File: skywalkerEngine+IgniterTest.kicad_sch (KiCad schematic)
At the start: 48 parts

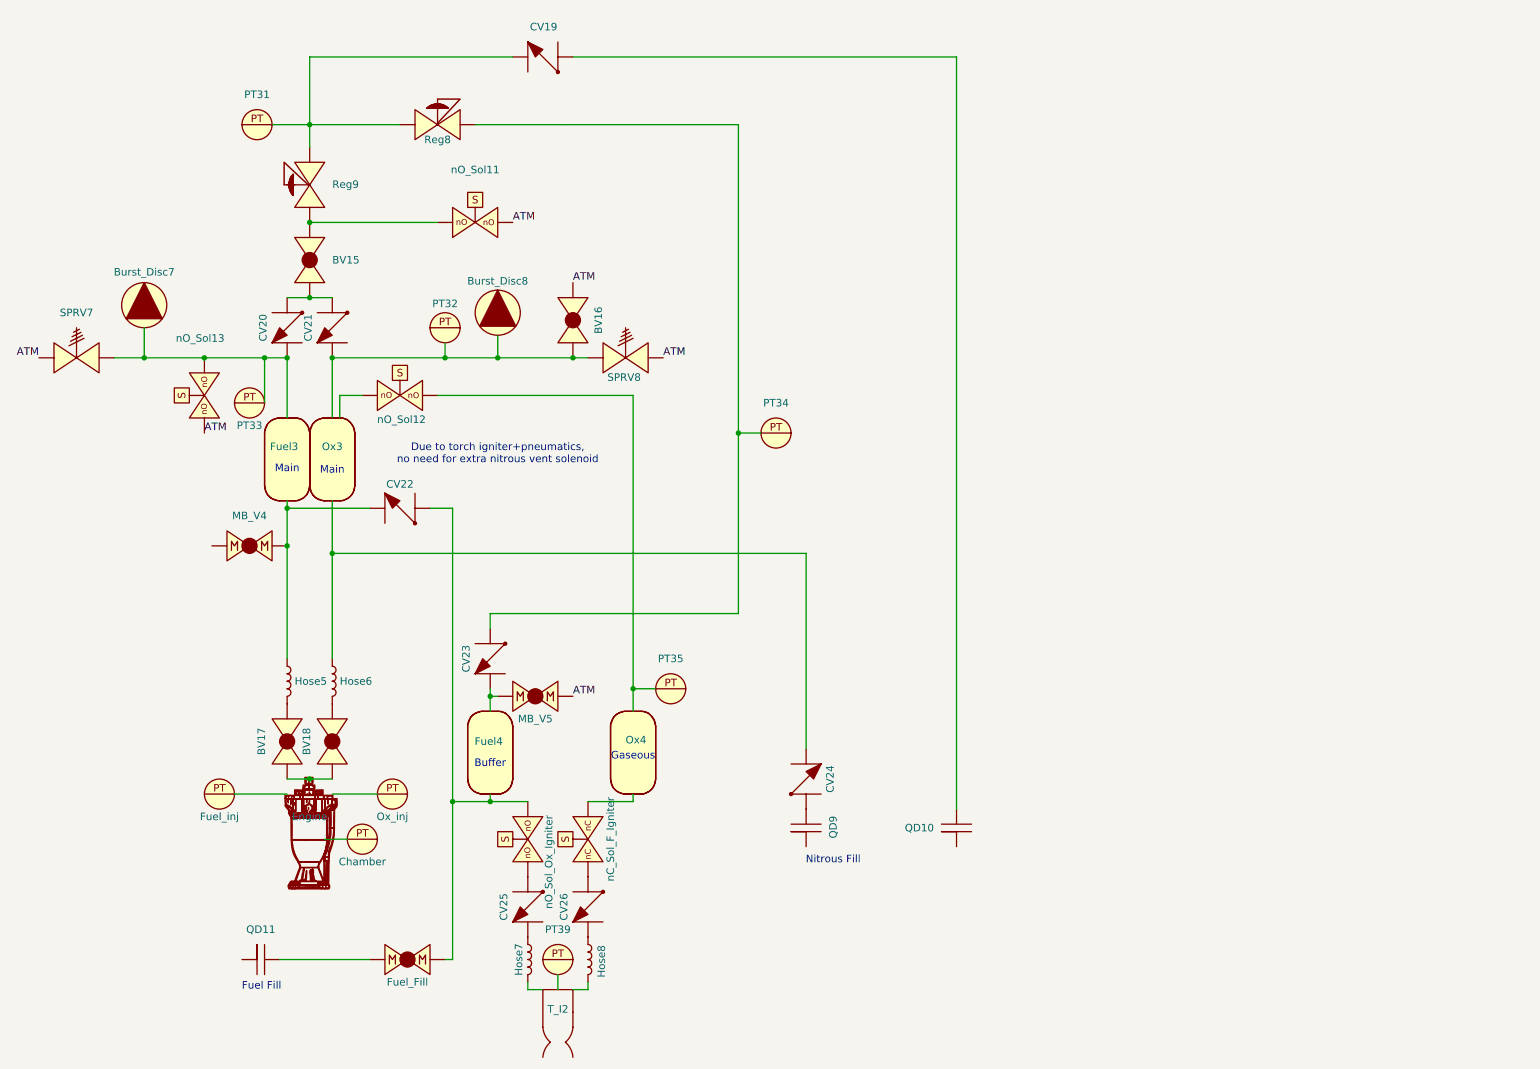
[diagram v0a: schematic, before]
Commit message: overwrite
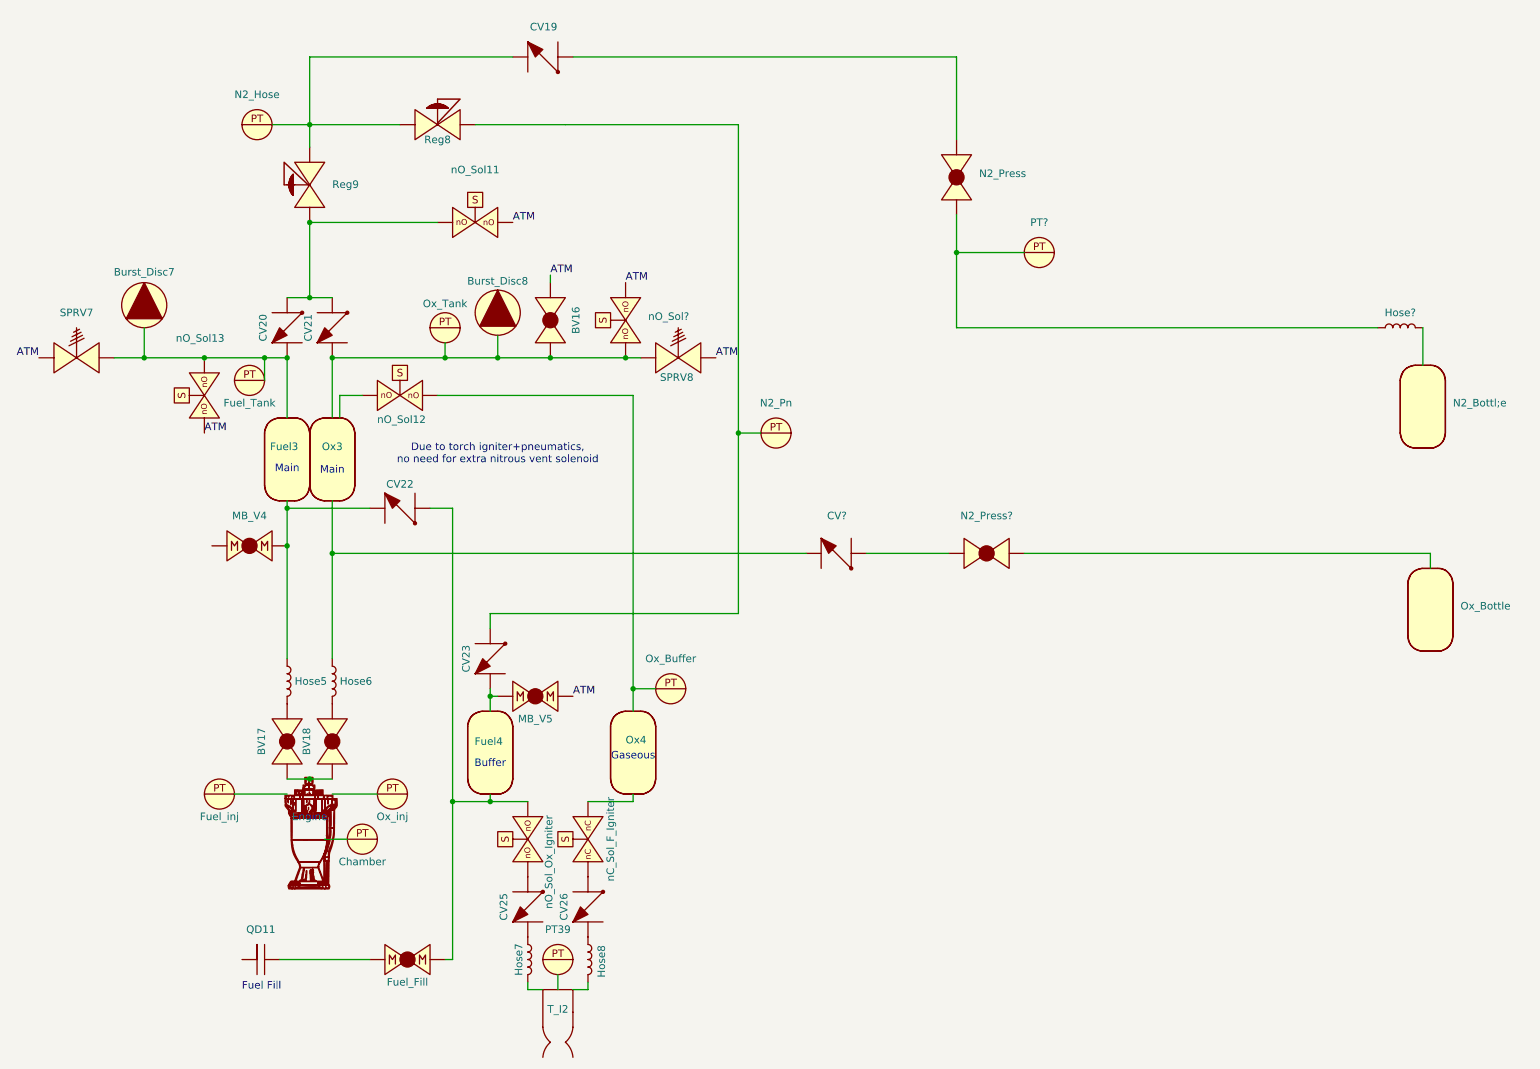
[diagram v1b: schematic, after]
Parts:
- removed BV15: ~, symbol PID_symbols:Ball_Valve
- removed CV24: ~, symbol PID_symbols:Check_Valve
- removed QD10, QD9: ~, symbol PID_symbols:Quick_Disconnect
- added CV?: ~, symbol PID_symbols:Check_Valve
- added Hose?: ~, symbol Device:Hose
- added N2_Bottl;e, Ox_Bottle: ~, symbol PID_symbols:Tank
- added N2_Press, N2_Press?: ~, symbol PID_symbols:Ball_Valve
- added PT?: ~, symbol PID_symbols:Pressure_Transducer
- added nO_Sol?: ~, symbol PID_symbols:Normally Open Solenoid
- renumbered PT33 to Fuel_Tank, PT31 to N2_Hose, PT34 to N2_Pn, PT35 to Ox_Buffer, PT32 to Ox_Tank
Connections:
- net ATM: now also nO_Sol?.
- net at Fuel_inj.: now also Engine.
- net at Engine.: now also Ox_inj.; no longer Fuel_inj.
- net at CV25.: now also Hose7.1; no longer nO_Sol_Ox_Igniter.
- net at CV20., CV21.: now also Reg9., nO_Sol11.
- net at MB_V4.: now also CV22., Fuel3., Hose5.1
- net at Reg9.: now also CV19., N2_Hose., Reg8.; no longer nO_Sol11.
- net at Hose6.1, Ox3.: now also CV?.
- net at Ox_inj.: no longer Engine.
- net at CV19.: now also N2_Press.
- new net: Burst_Disc7., CV20., Fuel3., Fuel_Tank., SPRV7., nO_Sol13.
- new net: Ox4., Ox_Buffer., nO_Sol12.
- new net: CV25., nO_Sol_Ox_Igniter.
- new net: CV23., N2_Pn., Reg8.
- new net: CV23., Fuel4., MB_V5.
- new net: Hose?.1, N2_Press., PT?.
- new net: BV17., BV18., Engine.
- new net: BV16., Burst_Disc8., CV21., Ox3., Ox_Tank., SPRV8., nO_Sol?.
- new net: N2_Press?., Ox_Bottle.
- new net: Hose?.2, N2_Bottl;e.
- new net: CV?., N2_Press?.
- now unconnected: Burst_Disc7., Burst_Disc8., Fuel_Tank., N2_Pn., Ox_Buffer., Ox_Tank.
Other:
- note removed: "Nitrous Fill"
- moved on the sheet: BV16, Fuel_Tank, SPRV8

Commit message: no message
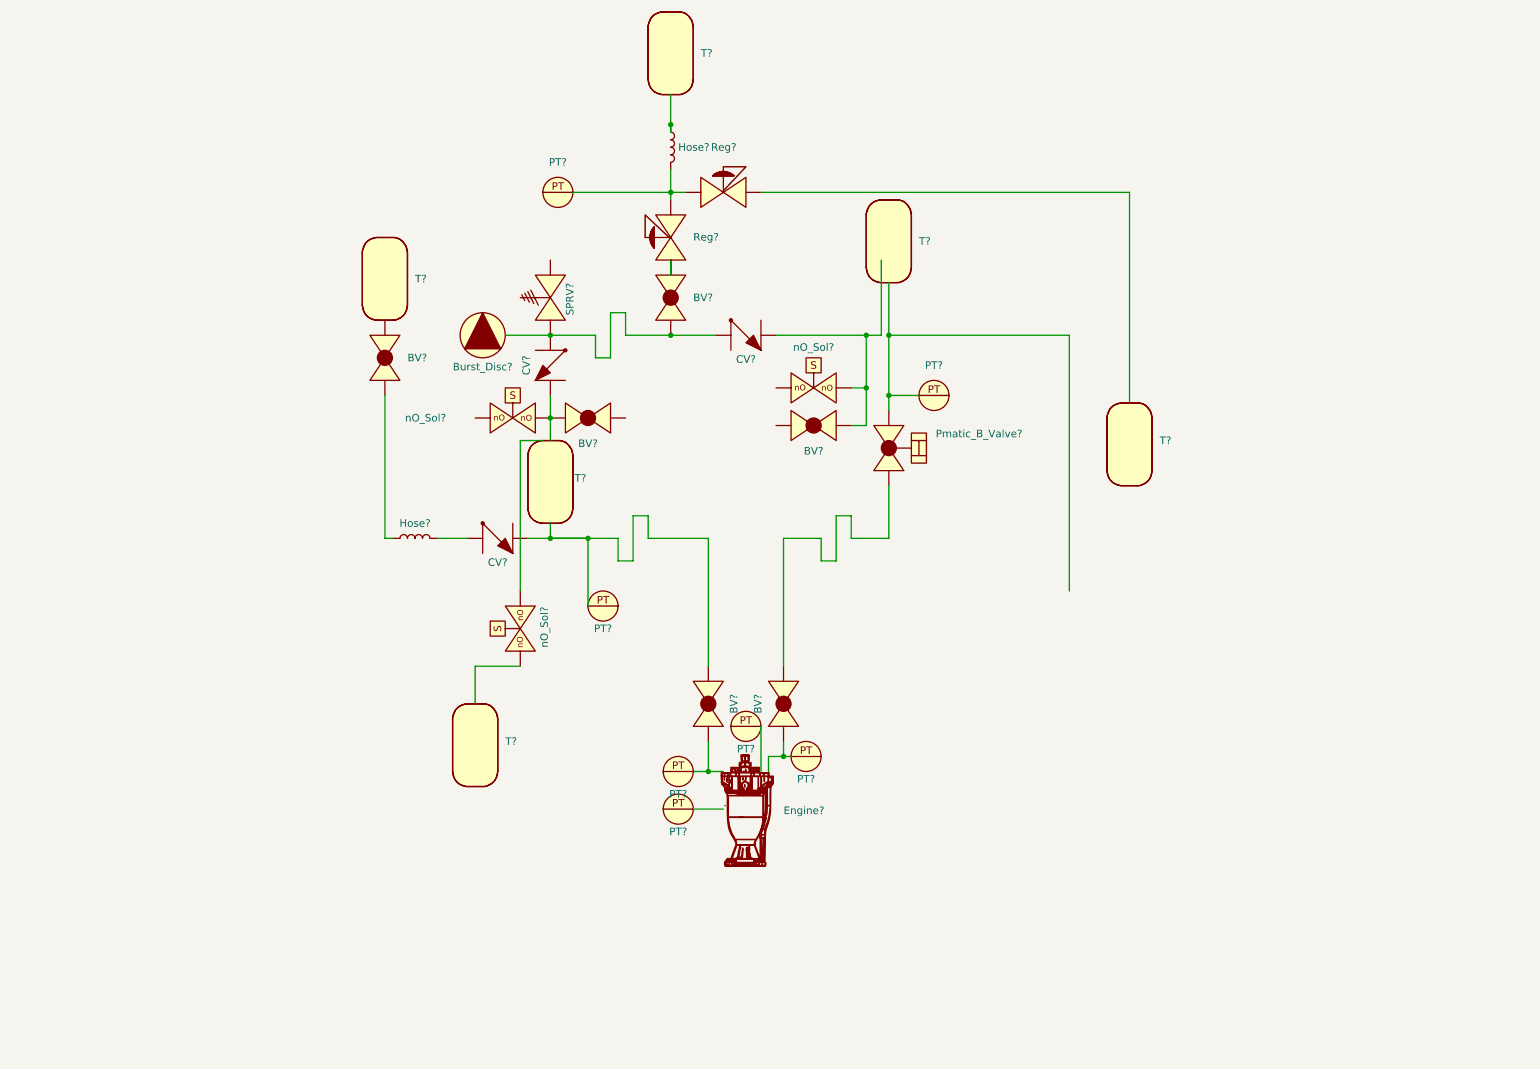
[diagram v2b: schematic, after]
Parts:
- removed BV16, BV17, BV18, N2_Press, N2_Press?: ~, symbol PID_symbols:Ball_Valve
- removed Burst_Disc7, Burst_Disc8: ~, symbol PID_symbols:Burst_Disc
- removed CV19, CV20, CV21, CV22, CV23, CV25, CV26, CV?: ~, symbol PID_symbols:Check_Valve
- removed Chamber, Fuel_Tank, Fuel_inj, N2_Hose, N2_Pn, Ox_Buffer, Ox_Tank, Ox_inj, PT39, PT?: ~, symbol PID_symbols:Pressure_Transducer
- removed Engine: ~, symbol PID_symbols:Engine
- removed Fuel3, Fuel4, N2_Bottl;e, Ox3, Ox4, Ox_Bottle: ~, symbol PID_symbols:Tank
- removed Fuel_Fill, MB_V4, MB_V5: ~, symbol PID_symbols:MBallValve
- removed Hose5, Hose6, Hose7, Hose8, Hose?: ~, symbol Device:Hose
- removed QD11: ~, symbol PID_symbols:Quick_Disconnect
- removed Reg8, Reg9: ~, symbol PID_symbols:Pressure_Regulator
- removed SPRV7, SPRV8: ~, symbol PID_symbols:SPRV
- removed T_I2: ~, symbol Analog_ADC:Torch_Igniter
- removed nC_Sol_F_Igniter: ~, symbol PID_symbols:Normally_Closed_Solenoid
- removed nO_Sol11, nO_Sol12, nO_Sol13, nO_Sol_Ox_Igniter: ~, symbol PID_symbols:Solenoid
- removed nO_Sol?: ~, symbol PID_symbols:Normally Open Solenoid
- added BV? (x6): ~, symbol PID_symbols:Ball_Valve
- added Burst_Disc?: ~, symbol PID_symbols:Burst_Disc
- added CV? (x3): ~, symbol PID_symbols:Check_Valve
- added Engine?: ~, symbol PID_symbols:Engine
- added Hose? (x2): ~, symbol Device:Hose
- added PT? (x7): ~, symbol PID_symbols:Pressure_Transducer
- added Pmatic_B_Valve?: ~, symbol PID_symbols:Pneumatic_Rotary_Ball_Valve
- added Reg? (x2): ~, symbol PID_symbols:Pressure_Regulator
- added SPRV?: ~, symbol PID_symbols:SPRV
- added T? (x6): ~, symbol PID_symbols:Tank
- added nO_Sol? (x3): ~, symbol PID_symbols:Solenoid
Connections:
- net .: now also PT?.
- new net: BV?., Engine?., PT?. (x2)
- new net: Reg?., T?.
- new net: BV?., Pmatic_B_Valve?.
- new net: BV?., CV?., PT?., T?.
- new net: CV?., Hose?.2
- new net: Hose?.1, T?.
- new net: BV?., Burst_Disc?., CV?., CV?., SPRV?.
- new net: BV?., Reg?.
- new net: T?., nO_Sol?.
- new net: BV?., CV?., T?., nO_Sol?.
- new net: BV?., T?.
- new net: Hose?.2, PT?., Reg?., Reg?.
- new net: PT?., Pmatic_B_Valve?., T?.
- new net: BV?., Hose?.1
- new net: BV?., CV?., nO_Sol?.
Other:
- note removed: "Buffer"
- note removed: "Due to torch igniter+pneumatics, no need for extra nitrous vent solenoid"
- note removed: "Fuel Fill"
- note removed: "Gaseous"
- note removed: "Main"

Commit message: no message
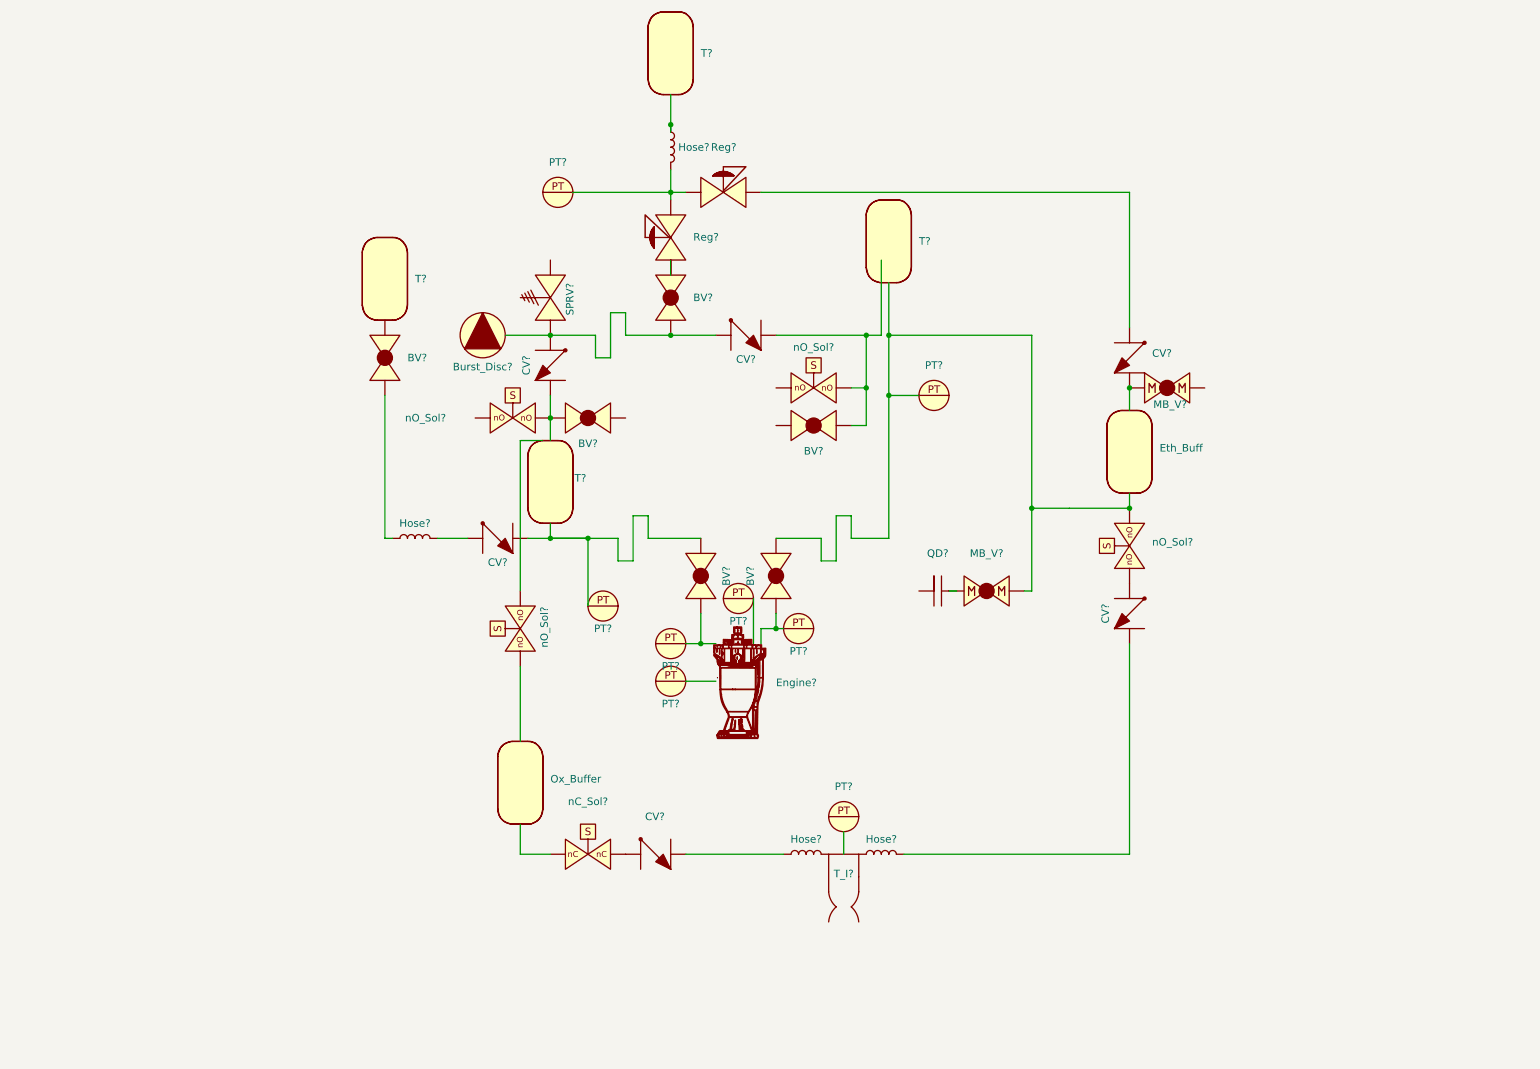
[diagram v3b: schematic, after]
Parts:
- removed Pmatic_B_Valve?: ~, symbol PID_symbols:Pneumatic_Rotary_Ball_Valve
- added CV? (x3): ~, symbol PID_symbols:Check_Valve
- added Hose? (x2): ~, symbol Device:Hose
- added MB_V? (x2): ~, symbol PID_symbols:MBallValve
- added PT?: ~, symbol PID_symbols:Pressure_Transducer
- added QD?: ~, symbol PID_symbols:Quick_Disconnect
- added T_I?: ~, symbol Analog_ADC:Torch_Igniter
- added nC_Sol?: ~, symbol PID_symbols:Normally_Closed_Solenoid
- added nO_Sol?: ~, symbol PID_symbols:Normally Open Solenoid
- gave numbers to parts that had none: 2
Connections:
- net at Engine?.: now also BV?., PT?.
- net at Eth_Buff.: now also BV?., PT?., T?., MB_V?., nO_Sol?.
- net at Reg?.: now also CV?.; no longer Eth_Buff.
- net at T?.: now also Hose?.1
- net at nO_Sol?.: now also Ox_Buffer.
- net at BV?.: now also CV?., T?., nO_Sol?.
- net at T?.: now also BV?.
- net at BV?.: now also Hose?.1; no longer T?.
- net at PT?.: no longer T?.
- net at BV?.: now also CV?., nO_Sol?.
- new net: BV?., Engine?., PT?.
- new net: CV?., Eth_Buff., MB_V?.
- new net: CV?., nC_Sol?.
- new net: Ox_Buffer., nC_Sol?.
- new net: BV?., CV?., PT?., T?.
- new net: BV?., Burst_Disc?., CV?., CV?., SPRV?.
- new net: CV?., Hose?.1
- new net: Hose?.2, T_I?.
- new net: CV?., nO_Sol?.
- new net: CV?., Hose?.2
- new net: MB_V?., QD?.
- new net: Hose?.1, T_I?.
- now unconnected: Burst_Disc?., PT?., PT?., PT?., SPRV?., nO_Sol?., nO_Sol?.
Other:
- moved on the sheet: BV?, Engine?, Eth_Buff, Ox_Buffer, PT?

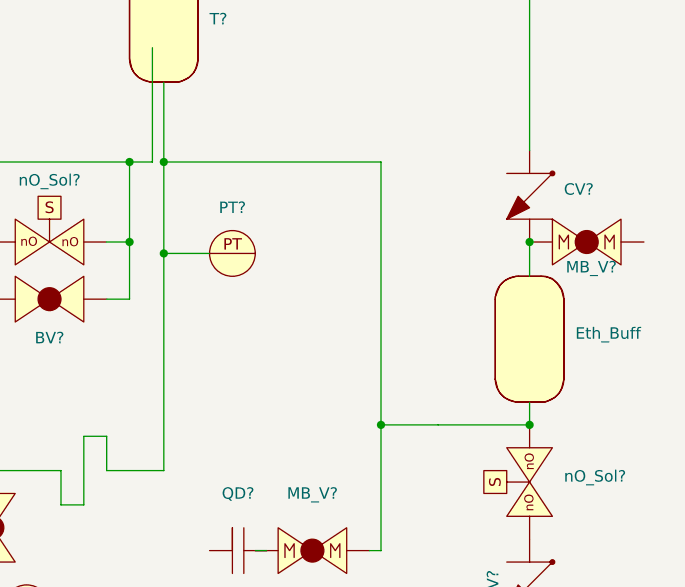
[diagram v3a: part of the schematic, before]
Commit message: no message
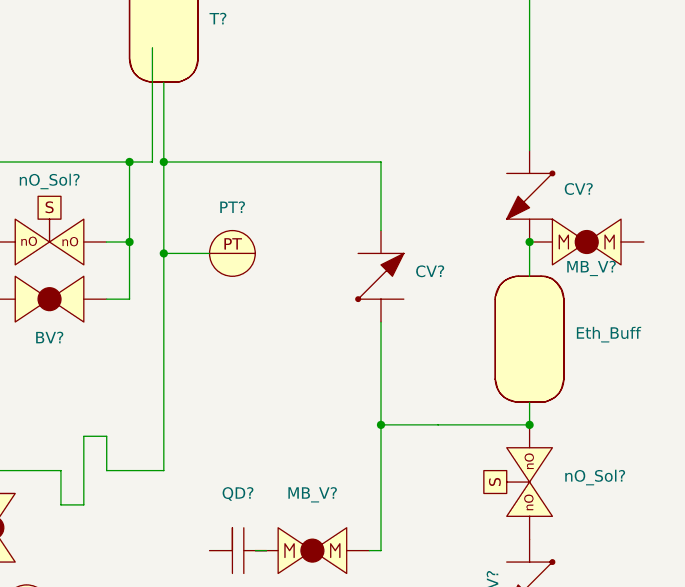
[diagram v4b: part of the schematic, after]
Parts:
- added CV?: ~, symbol PID_symbols:Check_Valve
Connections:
- net at Engine?.: now also BV?., PT?.
- net at nC_Sol?.: now also Ox_Buffer.; no longer CV?.
- net at Ox_Buffer.: now also nO_Sol?.; no longer nC_Sol?.
- net at T?.: now also Hose?.1
- net at BV?.: now also CV?., T?., nO_Sol?.
- net at T?.: now also BV?.
- net at BV?.: now also Hose?.1; no longer T?.
- net at QD?.: now also MB_V?.
- net at BV?.: now also CV?., nO_Sol?.
- new net: CV?., Eth_Buff., MB_V?., nO_Sol?.
- new net: BV?., CV?., PT?., T?. (x2)
- new net: BV?., Engine?., PT?.
- new net: CV?., Eth_Buff., MB_V?.
- new net: CV?., nC_Sol?.
- new net: BV?., Burst_Disc?., CV?., CV?., SPRV?.
- now unconnected: Burst_Disc?., MB_V?., PT?., PT?., PT?., PT?., SPRV?., T?., nO_Sol?., nO_Sol?.
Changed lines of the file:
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@@
+	(wire
+		(pts
+			(xy 186.69 91.44) (xy 186.69 102.87)
+		)
+		(stroke
+			(width 0.635)
+			(type default)
+		)
+	)
 	(wire
 		(pts
@@
 	(wire
 		(pts
-			(xy 186.69 73.66) (xy 186.69 102.87)
+			(xy 186.69 73.66) (xy 186.69 81.28)
 		)
 		(stroke
@@
 		)
 	)
+	(symbol
+		(lib_name "Check_Valve_3")
+		(lib_id "PID_symbols:Check_Valve")
+		(at 186.69 88.9 90)
+		(unit 1)
+		(exclude_from_sim no)
+		(in_bom yes)
+		(on_board yes)
+		(dnp no)
+		(fields_autoplaced yes)
+		(property "Reference" "CV?"
+			(at 190.5 85.8519 90)
+			(effects
+				(font
+					(size 1.27 1.27)
+				)
+				(justify right)
+			)
+		)
+		(property "Value" "~"
+			(at 190.5 87.757 90)
+			(effects
+				(font
+					(size 1.27 1.27)
+				)
+				(justify right)
+			)
+		)
+		(property "Footprint" ""
+			(at 186.69 88.9 0)
+			(effects
+				(font
+					(size 1.27 1.27)
+				)
+				(hide yes)
+			)
+		)
+		(property "Datasheet" ""
+			(at 186.69 88.9 0)
+			(effects
+				(font
+					(size 1.27 1.27)
+				)
+				(hide yes)
+			)
+		)
+		(property "Description" ""
+			(at 186.69 88.9 0)
+			(effects
+				(font
+					(size 1.27 1.27)
+				)
+				(hide yes)
+			)
+		)
+		(pin ""
+		)
+		(pin ""
+		)
+		(instances
+			(project ""
+				(path "/045f1f05-3134-4b6d-91b6-463031104f1e/e56eb7fc-ceaa-4516-b7d6-446a7aeba6c0"
+					(reference "CV?")
+					(unit 1)
+				)
+			)
+		)
+	)
